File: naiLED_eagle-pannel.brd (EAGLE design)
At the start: 79.5 x 97.8 mm, 378 parts, among them IC1 TCS3414, IC10 TCS3414, IC11 TCS3414, IC12 TCS3414, IC13 TCS3414, IC14 TCS3414, IC15 TCS3414, IC16 TCS3414, IC17 TCS3414, IC18 TCS3414, IC19 TCS3414, IC2 TCS3414, IC20 TCS3414, IC21 TCS3414, IC22 TCS3414, IC23 TCS3414, IC24 TCS3414, IC25 TCS3414, IC26 TCS3414, IC27 TCS3414, IC28 TCS3414, IC29 TCS3414, IC3 TCS3414, IC30 TCS3414, IC31 TCS3414, IC32 TCS3414, IC33 TCS3414, IC34 TCS3414, IC35 TCS3414, IC36 TCS3414, IC37 TCS3414, IC38 TCS3414, IC39 TCS3414, IC4 TCS3414, IC40 TCS3414, IC41 TCS3414, IC42 TCS3414, IC5 TCS3414, IC6 TCS3414, IC7 TCS3414, IC8 TCS3414, IC9 TCS3414, U1 24LC00T-I/OT, U10 ATTINY25-20SSU, U11 24LC00T-I/OT, U12 ATTINY25-20SSU, U13 24LC00T-I/OT, U14 ATTINY25-20SSU, U15 24LC00T-I/OT, U16 ATTINY25-20SSU, U17 24LC00T-I/OT, U18 ATTINY25-20SSU, U19 24LC00T-I/OT, U2 24LC00T-I/OT, U20 ATTINY25-20SSU, U21 24LC00T-I/OT, U22 ATTINY25-20SSU, U23 24LC00T-I/OT, U24 ATTINY25-20SSU, U25 24LC00T-I/OT, U26 ATTINY25-20SSU, U27 24LC00T-I/OT, U28 ATTINY25-20SSU, U29 24LC00T-I/OT, U3 ATTINY25-20SSU, U30 ATTINY25-20SSU, U31 24LC00T-I/OT, U32 ATTINY25-20SSU, U33 24LC00T-I/OT, U34 ATTINY25-20SSU, U35 24LC00T-I/OT, U36 ATTINY25-20SSU, U37 24LC00T-I/OT, U38 ATTINY25-20SSU, U39 24LC00T-I/OT, U4 ATTINY25-20SSU, U40 ATTINY25-20SSU, U41 24LC00T-I/OT, U42 ATTINY25-20SSU, U43 24LC00T-I/OT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

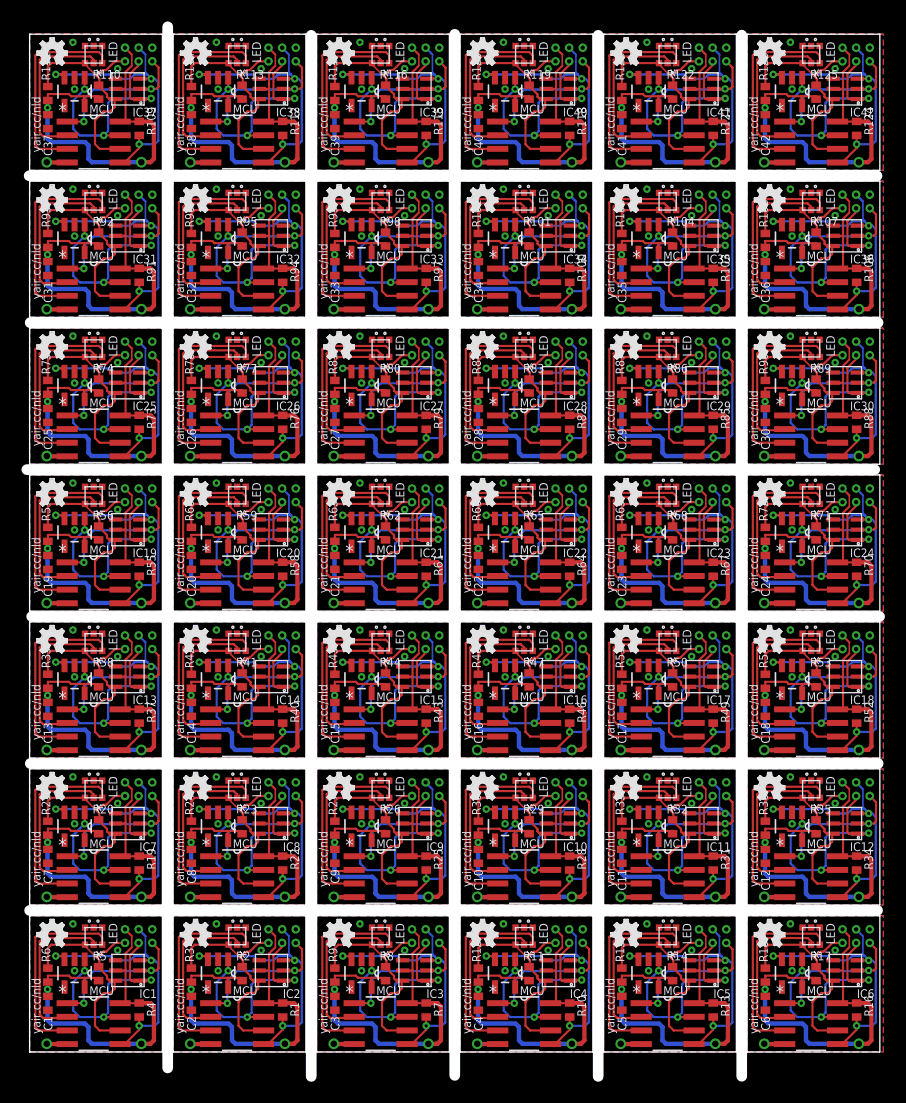
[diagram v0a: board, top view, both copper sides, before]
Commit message: auditing
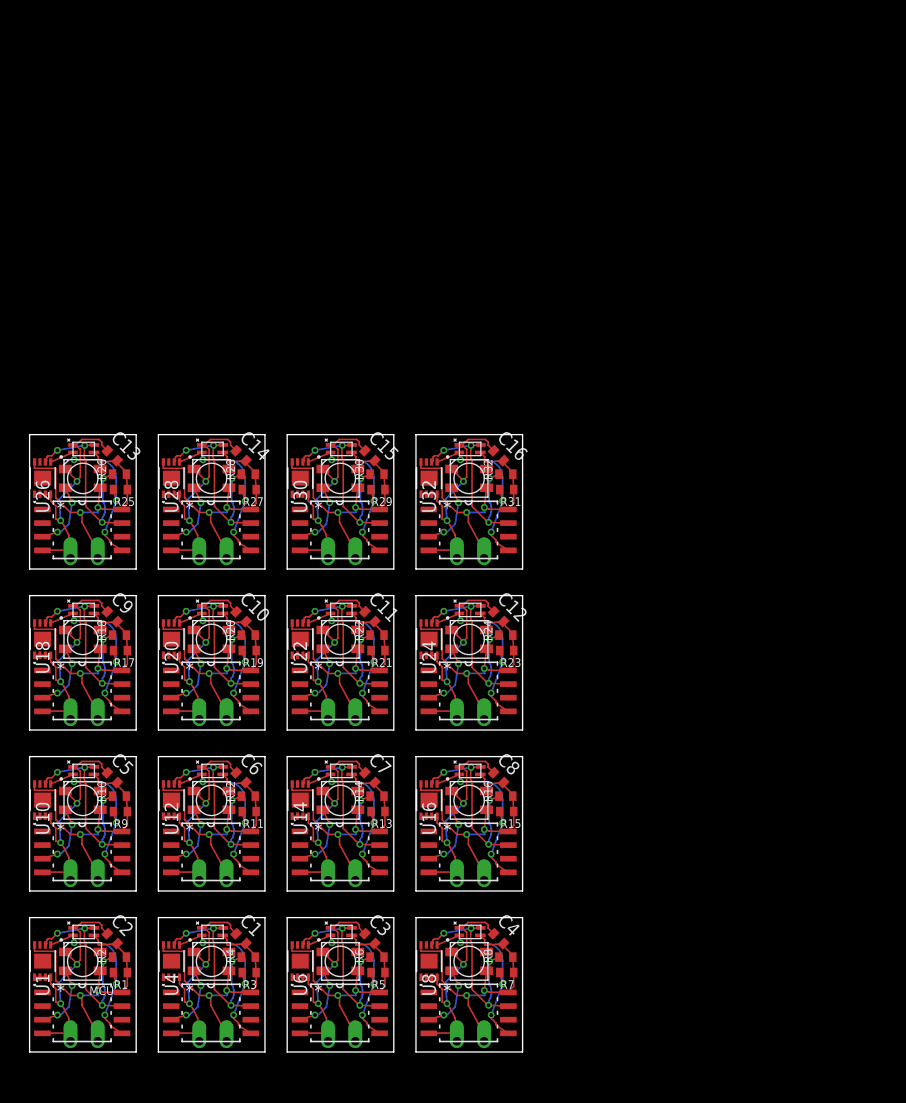
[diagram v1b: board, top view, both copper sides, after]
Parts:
- removed C17, C18, C19, C20, C21, C22, C23, C24, C25, C26, C27, C28, C29, C30, C31, C32, C33, C34, C35, C36, C37, C38, C39, C40, C41, C42: (no value), dp_devices:C402
- removed E$17, E$18, E$19, E$20, E$21, E$22, E$23, E$24, E$25, E$26, E$27, E$28, E$29, E$30, E$31, E$32, E$33, E$34, E$35, E$36, E$37, E$38, E$39, E$40, E$41, E$42: (no value), Logo:OSHW_FILLX100_NOTEXT
- removed IC1, IC10, IC11, IC12, IC13, IC14, IC15, IC16, IC17, IC18, IC19, IC2, IC20, IC21, IC22, IC23, IC24, IC25, IC26, IC27, IC28, IC29, IC3, IC30, IC31, IC32, IC33, IC34, IC35, IC36, IC37, IC38, IC39, IC4, IC40, IC41, IC42, IC5, IC6, IC7, IC8, IC9: TCS3414, yair_r:DFN-6PIN
- removed LED1, LED10, LED11, LED12, LED13, LED14, LED15, LED16, LED17, LED18, LED19, LED2, LED20, LED21, LED22, LED23, LED24, LED25, LED26, LED27, LED28, LED29, LED3, LED30, LED31, LED32, LED33, LED34, LED35, LED36, LED37, LED38, LED39, LED4, LED40, LED41, LED42, LED5, LED6, LED7, LED8, LED9: LED_RGB3, dp_devices:RGBLED
- removed R100, R101, R102, R103, R104, R105, R106, R107, R108, R109, R110, R111, R112, R113, R114, R115, R116, R117, R118, R119, R120, R121, R122, R123, R124, R125, R126, R33, R34, R35, R36, R37, R38, R39, R40, R41, R42, R43, R44, R45, R46, R47, R48, R49, R50, R51, R52, R53, R54, R55, R56, R57, R58, R59, R60, R61, R62, R63, R64, R65, R66, R67, R68, R69, R70, R71, R72, R73, R74, R75, R76, R77, R78, R79, R80, R81, R82, R83, R84, R85, R86, R87, R88, R89, R90, R91, R92, R93, R94, R95, R96, R97, R98, R99: (no value), dp_devices:R402
- removed U33, U35, U37, U39, U41, U43, U45, U47, U49, U51, U53, U55, U57, U59, U61, U63, U65, U67, U69, U71, U73, U75, U77, U79, U81, U83: 24LC00T-I/OT, Microchip-24LCxxx:SOT95P290X145-5N
- removed U34, U36, U38, U40, U42, U44, U46, U48, U50, U52, U54, U56, U58, U60, U62, U64, U66, U68, U70, U72, U74, U76, U78, U80, U82, U84: ATTINY25-20SSU, yair_r:SOIC127P600X175-8N
- added U$1, U$10, U$13, U$16, U$19, U$22, U$25, U$28, U$31, U$34, U$37, U$4, U$40, U$43, U$46, U$7: SK6812MINI, naiLED_eagle:LED-3535
- added U$11, U$14, U$17, U$2, U$20, U$23, U$26, U$29, U$32, U$35, U$38, U$41, U$44, U$47, U$5, U$8: VEML6040, naiLED_eagle:4-TFLGA
- added U$12, U$15, U$18, U$21, U$24, U$27, U$3, U$30, U$33, U$36, U$39, U$42, U$45, U$48, U$6, U$9, VCC, VCC1, VCC10, VCC11, VCC12, VCC13, VCC14, VCC15, VCC2, VCC3, VCC4, VCC5, VCC6, VCC7, VCC8, VCC9: HEADER-1X1, naiLED_eagle:1X1_LONG
- C1, C10, C11, C12, C13, C14, C15, C16, C2, C3, C4, C5, C6, C7, C8, C9: device dp_devices:C402 -> naiLED_eagle:C402
- R1, R10, R11, R12, R13, R14, R15, R16, R17, R18, R19, R2, R20, R21, R22, R23, R24, R25, R26, R27, R28, R29, R3, R30, R31, R32, R4, R5, R6, R7, R8, R9: device dp_devices:R402 -> naiLED_eagle:R402
- U1: value 24LC00T-I/OT -> AT24C256C-MAHL-T; device Microchip-24LCxxx:SOT95P290X145-5N -> naiLED_eagle:8MA2
- U10, U12, U14, U16, U18, U20, U22, U24, U26, U28, U30, U32, U4, U6, U8: value ATTINY25-20SSU -> AT24C256C-MAHL-T; device yair_r:SOIC127P600X175-8N -> naiLED_eagle:8MA2
- U11, U13, U15, U17, U19, U2, U21, U23, U25, U27, U29, U31, U5, U7, U9: value 24LC00T-I/OT -> ATTINY85-20SU; device Microchip-24LCxxx:SOT95P290X145-5N -> naiLED_eagle:SOIC127P798X216-8N
- U3: value ATTINY25-20SSU -> ATTINY85-20SU; device yair_r:SOIC127P600X175-8N -> naiLED_eagle:SOIC127P798X216-8N
- moved R17 71.5 mm to (8.46, 37.4), turned to 0 degrees
- moved R18 68.0 mm to (8.37, 38.8), turned to 0 degrees
- moved U12 63.1 mm to (13.2, 23.5), turned to 90 degrees
- moved U10 61.8 mm to (1.22, 23.5), turned to 90 degrees
- moved U11 55.3 mm to (16.9, 18.6), turned to 0 degrees
- moved U9 54.0 mm to (4.90, 18.6), turned to 0 degrees
- moved C6 53.2 mm to (19.7, 25.6), turned to 315 degrees
- moved C5 51.9 mm to (7.70, 25.6), turned to 315 degrees
- moved E$6 50.8 mm to (18.3, 22.5), flipped to the bottom
- moved E$5 49.5 mm to (6.32, 22.5), flipped to the bottom
- moved R28 47.0 mm to (20.4, 53.8), turned to 0 degrees
- moved R10 46.4 mm to (8.37, 23.8), turned to 0 degrees
- moved R25 45.0 mm to (8.46, 52.4), turned to 0 degrees
- moved U24 41.9 mm to (37.2, 38.5), turned to 90 degrees
- moved R26 41.2 mm to (8.37, 53.8), turned to 0 degrees
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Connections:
- removed net D0/PWM/MOSI/SDA16: IC17.P$3, R49.1, U33.3, U34.5
- removed net D0/PWM/MOSI/SDA17: IC18.P$3, R52.1, U35.3, U36.5
- removed net D0/PWM/MOSI/SDA18: IC19.P$3, R55.1, U37.3, U38.5
- removed net D0/PWM/MOSI/SDA19: IC20.P$3, R58.1, U39.3, U40.5
- removed net D0/PWM/MOSI/SDA20: IC21.P$3, R61.1, U41.3, U42.5
- removed net D0/PWM/MOSI/SDA21: IC22.P$3, R64.1, U43.3, U44.5
- removed net D0/PWM/MOSI/SDA22: IC23.P$3, R67.1, U45.3, U46.5
- removed net D0/PWM/MOSI/SDA23: IC24.P$3, R70.1, U47.3, U48.5
- removed net D0/PWM/MOSI/SDA24: IC25.P$3, R73.1, U49.3, U50.5
- removed net D0/PWM/MOSI/SDA25: IC26.P$3, R76.1, U51.3, U52.5
- removed net D0/PWM/MOSI/SDA26: IC27.P$3, R79.1, U53.3, U54.5
- removed net D0/PWM/MOSI/SDA27: IC28.P$3, R82.1, U55.3, U56.5
- removed net D0/PWM/MOSI/SDA28: IC29.P$3, R85.1, U57.3, U58.5
- removed net D0/PWM/MOSI/SDA29: IC30.P$3, R88.1, U59.3, U60.5
- removed net D0/PWM/MOSI/SDA30: IC31.P$3, R91.1, U61.3, U62.5
- removed net D0/PWM/MOSI/SDA31: IC32.P$3, R94.1, U63.3, U64.5
- removed net D0/PWM/MOSI/SDA32: IC33.P$3, R97.1, U65.3, U66.5
- removed net D0/PWM/MOSI/SDA33: IC34.P$3, R100.1, U67.3, U68.5
- removed net D0/PWM/MOSI/SDA34: IC35.P$3, R103.1, U69.3, U70.5
- removed net D0/PWM/MOSI/SDA35: IC36.P$3, R106.1, U71.3, U72.5
- removed net D0/PWM/MOSI/SDA36: IC37.P$3, R109.1, U73.3, U74.5
- removed net D0/PWM/MOSI/SDA37: IC38.P$3, R112.1, U75.3, U76.5
- removed net D0/PWM/MOSI/SDA38: IC39.P$3, R115.1, U77.3, U78.5
- removed net D0/PWM/MOSI/SDA39: IC40.P$3, R118.1, U79.3, U80.5
- removed net D0/PWM/MOSI/SDA40: IC41.P$3, R121.1, U81.3, U82.5
- removed net D0/PWM/MOSI/SDA41: IC42.P$3, R124.1, U83.3, U84.5
- removed net D1/PWM/MISO16: IC17.P$4, LED17.AG, R50.1, R51.2, U34.6
- removed net D1/PWM/MISO17: IC18.P$4, LED18.AG, R53.1, R54.2, U36.6
- removed net D1/PWM/MISO18: IC19.P$4, LED19.AG, R56.1, R57.2, U38.6
- removed net D1/PWM/MISO19: IC20.P$4, LED20.AG, R59.1, R60.2, U40.6
- removed net D1/PWM/MISO20: IC21.P$4, LED21.AG, R62.1, R63.2, U42.6
- removed net D1/PWM/MISO21: IC22.P$4, LED22.AG, R65.1, R66.2, U44.6
- removed net D1/PWM/MISO22: IC23.P$4, LED23.AG, R68.1, R69.2, U46.6
- removed net D1/PWM/MISO23: IC24.P$4, LED24.AG, R71.1, R72.2, U48.6
- removed net D1/PWM/MISO24: IC25.P$4, LED25.AG, R74.1, R75.2, U50.6
- removed net D1/PWM/MISO25: IC26.P$4, LED26.AG, R77.1, R78.2, U52.6
- removed net D1/PWM/MISO26: IC27.P$4, LED27.AG, R80.1, R81.2, U54.6
- removed net D1/PWM/MISO27: IC28.P$4, LED28.AG, R83.1, R84.2, U56.6
- removed net D1/PWM/MISO28: IC29.P$4, LED29.AG, R86.1, R87.2, U58.6
- removed net D1/PWM/MISO29: IC30.P$4, LED30.AG, R89.1, R90.2, U60.6
- removed net D1/PWM/MISO30: IC31.P$4, LED31.AG, R92.1, R93.2, U62.6
- removed net D1/PWM/MISO31: IC32.P$4, LED32.AG, R95.1, R96.2, U64.6
- removed net D1/PWM/MISO32: IC33.P$4, LED33.AG, R98.1, R99.2, U66.6
- removed net D1/PWM/MISO33: IC34.P$4, LED34.AG, R101.1, R102.2, U68.6
- removed net D1/PWM/MISO34: IC35.P$4, LED35.AG, R104.1, R105.2, U70.6
- removed net D1/PWM/MISO35: IC36.P$4, LED36.AG, R107.1, R108.2, U72.6
- removed net D1/PWM/MISO36: IC37.P$4, LED37.AG, R110.1, R111.2, U74.6
- removed net D1/PWM/MISO37: IC38.P$4, LED38.AG, R113.1, R114.2, U76.6
- removed net D1/PWM/MISO38: IC39.P$4, LED39.AG, R116.1, R117.2, U78.6
- removed net D1/PWM/MISO39: IC40.P$4, LED40.AG, R119.1, R120.2, U80.6
- removed net D1/PWM/MISO40: IC41.P$4, LED41.AG, R122.1, R123.2, U82.6
- removed net D1/PWM/MISO41: IC42.P$4, LED42.AG, R125.1, R126.2, U84.6
- removed net D2/A1/SCK/SCL16: IC17.P$1, U33.1, U34.7
- removed net D2/A1/SCK/SCL17: IC18.P$1, U35.1, U36.7
- removed net D2/A1/SCK/SCL18: IC19.P$1, U37.1, U38.7
- removed net D2/A1/SCK/SCL19: IC20.P$1, U39.1, U40.7
- removed net D2/A1/SCK/SCL20: IC21.P$1, U41.1, U42.7
- removed net D2/A1/SCK/SCL21: IC22.P$1, U43.1, U44.7
- removed net D2/A1/SCK/SCL22: IC23.P$1, U45.1, U46.7
- removed net D2/A1/SCK/SCL23: IC24.P$1, U47.1, U48.7
- removed net D2/A1/SCK/SCL24: IC25.P$1, U49.1, U50.7
- removed net D2/A1/SCK/SCL25: IC26.P$1, U51.1, U52.7
- removed net D2/A1/SCK/SCL26: IC27.P$1, U53.1, U54.7
- removed net D2/A1/SCK/SCL27: IC28.P$1, U55.1, U56.7
- removed net D2/A1/SCK/SCL28: IC29.P$1, U57.1, U58.7
- removed net D2/A1/SCK/SCL29: IC30.P$1, U59.1, U60.7
- removed net D2/A1/SCK/SCL30: IC31.P$1, U61.1, U62.7
- removed net D2/A1/SCK/SCL31: IC32.P$1, U63.1, U64.7
- removed net D2/A1/SCK/SCL32: IC33.P$1, U65.1, U66.7
- removed net D2/A1/SCK/SCL33: IC34.P$1, U67.1, U68.7
- removed net D2/A1/SCK/SCL34: IC35.P$1, U69.1, U70.7
- removed net D2/A1/SCK/SCL35: IC36.P$1, U71.1, U72.7
- removed net D2/A1/SCK/SCL36: IC37.P$1, U73.1, U74.7
- removed net D2/A1/SCK/SCL37: IC38.P$1, U75.1, U76.7
- removed net D2/A1/SCK/SCL38: IC39.P$1, U77.1, U78.7
- removed net D2/A1/SCK/SCL39: IC40.P$1, U79.1, U80.7
- removed net D2/A1/SCK/SCL40: IC41.P$1, U81.1, U82.7
- removed net D2/A1/SCK/SCL41: IC42.P$1, U83.1, U84.7
- removed net D3/A17: LED17.AR, U34.2
- removed net D3/A18: LED18.AR, U36.2
- removed net D3/A19: LED19.AR, U38.2
- removed net D3/A20: LED20.AR, U40.2
- removed net D3/A21: LED21.AR, U42.2
- removed net D3/A22: LED22.AR, U44.2
- removed net D3/A23: LED23.AR, U46.2
- removed net D3/A24: LED24.AR, U48.2
- removed net D3/A25: LED25.AR, U50.2
- removed net D3/A26: LED26.AR, U52.2
- removed net D3/A27: LED27.AR, U54.2
- removed net D3/A28: LED28.AR, U56.2
- removed net D3/A29: LED29.AR, U58.2
- removed net D3/A30: LED30.AR, U60.2
- removed net D3/A31: LED31.AR, U62.2
- removed net D3/A32: LED32.AR, U64.2
- removed net D3/A33: LED33.AR, U66.2
- removed net D3/A34: LED34.AR, U68.2
- removed net D3/A35: LED35.AR, U70.2
- removed net D3/A36: LED36.AR, U72.2
- removed net D3/A37: LED37.AR, U74.2
- removed net D3/A38: LED38.AR, U76.2
- removed net D3/A39: LED39.AR, U78.2
- removed net D3/A40: LED40.AR, U80.2
- removed net D3/A41: LED41.AR, U82.2
- removed net D3/A42: LED42.AR, U84.2
- removed net D4/PWM16: LED17.AB, U34.3
- removed net D4/PWM17: LED18.AB, U36.3
- removed net D4/PWM18: LED19.AB, U38.3
- removed net D4/PWM19: LED20.AB, U40.3
- removed net D4/PWM20: LED21.AB, U42.3
- removed net D4/PWM21: LED22.AB, U44.3
- removed net D4/PWM22: LED23.AB, U46.3
- removed net D4/PWM23: LED24.AB, U48.3
- removed net D4/PWM24: LED25.AB, U50.3
- removed net D4/PWM25: LED26.AB, U52.3
- removed net D4/PWM26: LED27.AB, U54.3
- removed net D4/PWM27: LED28.AB, U56.3
- removed net D4/PWM28: LED29.AB, U58.3
- removed net D4/PWM29: LED30.AB, U60.3
- removed net D4/PWM30: LED31.AB, U62.3
- removed net D4/PWM31: LED32.AB, U64.3
- removed net D4/PWM32: LED33.AB, U66.3
- removed net D4/PWM33: LED34.AB, U68.3
- removed net D4/PWM34: LED35.AB, U70.3
- removed net D4/PWM35: LED36.AB, U72.3
- removed net D4/PWM36: LED37.AB, U74.3
- removed net D4/PWM37: LED38.AB, U76.3
- removed net D4/PWM38: LED39.AB, U78.3
- removed net D4/PWM39: LED40.AB, U80.3
- removed net D4/PWM40: LED41.AB, U82.3
- removed net D4/PWM41: LED42.AB, U84.3
- removed net D5/A0/RESET: IC1.P$2, U3.1
- removed net D5/A0/RESET1: IC2.P$2, U4.1
- removed net D5/A0/RESET10: IC11.P$2, U22.1
- removed net D5/A0/RESET11: IC12.P$2, U24.1
- removed net D5/A0/RESET12: IC13.P$2, U26.1
- removed net D5/A0/RESET13: IC14.P$2, U28.1
- removed net D5/A0/RESET14: IC15.P$2, U30.1
- removed net D5/A0/RESET15: IC16.P$2, U32.1
- removed net D5/A0/RESET16: IC17.P$2, U34.1
- removed net D5/A0/RESET17: IC18.P$2, U36.1
- removed net D5/A0/RESET18: IC19.P$2, U38.1
- removed net D5/A0/RESET19: IC20.P$2, U40.1
- removed net D5/A0/RESET2: IC3.P$2, U6.1
- removed net D5/A0/RESET20: IC21.P$2, U42.1
- removed net D5/A0/RESET21: IC22.P$2, U44.1
- removed net D5/A0/RESET22: IC23.P$2, U46.1
- removed net D5/A0/RESET23: IC24.P$2, U48.1
- removed net D5/A0/RESET24: IC25.P$2, U50.1
- removed net D5/A0/RESET25: IC26.P$2, U52.1
- removed net D5/A0/RESET26: IC27.P$2, U54.1
- removed net D5/A0/RESET27: IC28.P$2, U56.1
- removed net D5/A0/RESET28: IC29.P$2, U58.1
- removed net D5/A0/RESET29: IC30.P$2, U60.1
- removed net D5/A0/RESET3: IC4.P$2, U8.1
- removed net D5/A0/RESET30: IC31.P$2, U62.1
- removed net D5/A0/RESET31: IC32.P$2, U64.1
- removed net D5/A0/RESET32: IC33.P$2, U66.1
- removed net D5/A0/RESET33: IC34.P$2, U68.1
- removed net D5/A0/RESET34: IC35.P$2, U70.1
- removed net D5/A0/RESET35: IC36.P$2, U72.1
- removed net D5/A0/RESET36: IC37.P$2, U74.1
- removed net D5/A0/RESET37: IC38.P$2, U76.1
- removed net D5/A0/RESET38: IC39.P$2, U78.1
- removed net D5/A0/RESET39: IC40.P$2, U80.1
- removed net D5/A0/RESET4: IC5.P$2, U10.1
- removed net D5/A0/RESET40: IC41.P$2, U82.1
- removed net D5/A0/RESET41: IC42.P$2, U84.1
- removed net D5/A0/RESET5: IC6.P$2, U12.1
- removed net D5/A0/RESET6: IC7.P$2, U14.1
- removed net D5/A0/RESET7: IC8.P$2, U16.1
- removed net D5/A0/RESET8: IC9.P$2, U18.1
- removed net D5/A0/RESET9: IC10.P$2, U20.1
- removed net GND16: C17.2, IC17.P$6, LED17.CB, LED17.CG, LED17.CR, U33.2, U34.4
- removed net GND17: C18.2, IC18.P$6, LED18.CB, LED18.CG, LED18.CR, U35.2, U36.4
- removed net GND18: C19.2, IC19.P$6, LED19.CB, LED19.CG, LED19.CR, U37.2, U38.4
- removed net GND19: C20.2, IC20.P$6, LED20.CB, LED20.CG, LED20.CR, U39.2, U40.4
- removed net GND20: C21.2, IC21.P$6, LED21.CB, LED21.CG, LED21.CR, U41.2, U42.4
- removed net GND21: C22.2, IC22.P$6, LED22.CB, LED22.CG, LED22.CR, U43.2, U44.4
- removed net GND22: C23.2, IC23.P$6, LED23.CB, LED23.CG, LED23.CR, U45.2, U46.4
- removed net GND23: C24.2, IC24.P$6, LED24.CB, LED24.CG, LED24.CR, U47.2, U48.4
- removed net GND24: C25.2, IC25.P$6, LED25.CB, LED25.CG, LED25.CR, U49.2, U50.4
- removed net GND25: C26.2, IC26.P$6, LED26.CB, LED26.CG, LED26.CR, U51.2, U52.4
- removed net GND26: C27.2, IC27.P$6, LED27.CB, LED27.CG, LED27.CR, U53.2, U54.4
- removed net GND27: C28.2, IC28.P$6, LED28.CB, LED28.CG, LED28.CR, U55.2, U56.4
- removed net GND28: C29.2, IC29.P$6, LED29.CB, LED29.CG, LED29.CR, U57.2, U58.4
- removed net GND29: C30.2, IC30.P$6, LED30.CB, LED30.CG, LED30.CR, U59.2, U60.4
- removed net GND30: C31.2, IC31.P$6, LED31.CB, LED31.CG, LED31.CR, U61.2, U62.4
- removed net GND31: C32.2, IC32.P$6, LED32.CB, LED32.CG, LED32.CR, U63.2, U64.4
- removed net GND32: C33.2, IC33.P$6, LED33.CB, LED33.CG, LED33.CR, U65.2, U66.4
- removed net GND33: C34.2, IC34.P$6, LED34.CB, LED34.CG, LED34.CR, U67.2, U68.4
- removed net GND34: C35.2, IC35.P$6, LED35.CB, LED35.CG, LED35.CR, U69.2, U70.4
- removed net GND35: C36.2, IC36.P$6, LED36.CB, LED36.CG, LED36.CR, U71.2, U72.4
- removed net GND36: C37.2, IC37.P$6, LED37.CB, LED37.CG, LED37.CR, U73.2, U74.4
- removed net GND37: C38.2, IC38.P$6, LED38.CB, LED38.CG, LED38.CR, U75.2, U76.4
- removed net GND38: C39.2, IC39.P$6, LED39.CB, LED39.CG, LED39.CR, U77.2, U78.4
- removed net GND39: C40.2, IC40.P$6, LED40.CB, LED40.CG, LED40.CR, U79.2, U80.4
- removed net GND40: C41.2, IC41.P$6, LED41.CB, LED41.CG, LED41.CR, U81.2, U82.4
- removed net GND41: C42.2, IC42.P$6, LED42.CB, LED42.CG, LED42.CR, U83.2, U84.4
- removed net VCC16: C17.1, IC17.P$5, R49.2, R50.2, R51.1, U33.5, U34.8
- removed net VCC17: C18.1, IC18.P$5, R52.2, R53.2, R54.1, U35.5, U36.8
- removed net VCC18: C19.1, IC19.P$5, R55.2, R56.2, R57.1, U37.5, U38.8
- removed net VCC19: C20.1, IC20.P$5, R58.2, R59.2, R60.1, U39.5, U40.8
- removed net VCC20: C21.1, IC21.P$5, R61.2, R62.2, R63.1, U41.5, U42.8
- removed net VCC21: C22.1, IC22.P$5, R64.2, R65.2, R66.1, U43.5, U44.8
- removed net VCC22: C23.1, IC23.P$5, R67.2, R68.2, R69.1, U45.5, U46.8
- removed net VCC23: C24.1, IC24.P$5, R70.2, R71.2, R72.1, U47.5, U48.8
- removed net VCC24: C25.1, IC25.P$5, R73.2, R74.2, R75.1, U49.5, U50.8
- removed net VCC25: C26.1, IC26.P$5, R76.2, R77.2, R78.1, U51.5, U52.8
- removed net VCC26: C27.1, IC27.P$5, R79.2, R80.2, R81.1, U53.5, U54.8
- removed net VCC27: C28.1, IC28.P$5, R82.2, R83.2, R84.1, U55.5, U56.8
- removed net VCC28: C29.1, IC29.P$5, R85.2, R86.2, R87.1, U57.5, U58.8
- removed net VCC29: C30.1, IC30.P$5, R88.2, R89.2, R90.1, U59.5, U60.8
- removed net VCC30: C31.1, IC31.P$5, R91.2, R92.2, R93.1, U61.5, U62.8
- removed net VCC31: C32.1, IC32.P$5, R94.2, R95.2, R96.1, U63.5, U64.8
- removed net VCC32: C33.1, IC33.P$5, R97.2, R98.2, R99.1, U65.5, U66.8
- removed net VCC33: C34.1, IC34.P$5, R100.2, R101.2, R102.1, U67.5, U68.8
- removed net VCC34: C35.1, IC35.P$5, R103.2, R104.2, R105.1, U69.5, U70.8
- removed net VCC35: C36.1, IC36.P$5, R106.2, R107.2, R108.1, U71.5, U72.8
- removed net VCC36: C37.1, IC37.P$5, R109.2, R110.2, R111.1, U73.5, U74.8
- removed net VCC37: C38.1, IC38.P$5, R112.2, R113.2, R114.1, U75.5, U76.8
- removed net VCC38: C39.1, IC39.P$5, R115.2, R116.2, R117.1, U77.5, U78.8
- removed net VCC39: C40.1, IC40.P$5, R118.2, R119.2, R120.1, U79.5, U80.8
- removed net VCC40: C41.1, IC41.P$5, R121.2, R122.2, R123.1, U81.5, U82.8
- removed net VCC41: C42.1, IC42.P$5, R124.2, R125.2, R126.1, U83.5, U84.8
- new net NC: U3.1
- new net NC1: U2.1
- new net NC10: U21.1
- new net NC11: U23.1
- new net NC12: U25.1
- new net NC13: U27.1
- new net NC14: U29.1
- new net NC15: U31.1
- new net NC2: U5.1
- new net NC3: U7.1
- new net NC4: U9.1
- new net NC5: U11.1
- new net NC6: U13.1
- new net NC7: U15.1
- new net NC8: U17.1
- new net NC9: U19.1
- net D0/PWM/MOSI/SDA: now also R1.1, U$2.2, U1.5; no longer IC1.P$3, R4.1, U2.3
- net D0/PWM/MOSI/SDA1: now also R3.1, U$5.2, U2.5; no longer IC2.P$3, R1.1, U1.3
- net D0/PWM/MOSI/SDA10: now also R21.1, U$32.2, U21.5; no longer IC11.P$3, R31.1, U21.3
- net D0/PWM/MOSI/SDA11: now also R23.1, U$35.2, U23.5; no longer IC12.P$3, R34.1, U23.3
- net D0/PWM/MOSI/SDA12: now also R25.1, U$38.2, U25.5; no longer IC13.P$3, R37.1, U25.3
- net D0/PWM/MOSI/SDA13: now also R27.1, U$41.2, U27.5; no longer IC14.P$3, R40.1, U27.3
- net D0/PWM/MOSI/SDA14: now also R29.1, U$44.2, U29.5; no longer IC15.P$3, R43.1, U29.3
- net D0/PWM/MOSI/SDA15: now also R31.1, U$47.2, U31.5; no longer IC16.P$3, R46.1, U31.3
- net D0/PWM/MOSI/SDA2: now also R5.1, U$8.2, U5.5; no longer IC3.P$3, R7.1, U5.3
- net D0/PWM/MOSI/SDA3: now also R7.1, U$11.2, U7.5; no longer IC4.P$3, R10.1, U7.3
- net D0/PWM/MOSI/SDA4: now also R9.1, U$14.2, U9.5; no longer IC5.P$3, R13.1, U9.3
- net D0/PWM/MOSI/SDA5: now also R11.1, U$17.2, U11.5; no longer IC6.P$3, R16.1, U11.3
- net D0/PWM/MOSI/SDA6: now also R13.1, U$20.2, U13.5; no longer IC7.P$3, R19.1, U13.3
- net D0/PWM/MOSI/SDA7: now also R15.1, U$23.2, U15.5; no longer IC8.P$3, R22.1, U15.3
- net D0/PWM/MOSI/SDA8: now also R17.1, U$26.2, U17.5; no longer IC9.P$3, R25.1, U17.3
- net D0/PWM/MOSI/SDA9: now also R19.1, U$29.2, U19.5; no longer IC10.P$3, R28.1, U19.3
- net D1/PWM/MISO: no longer IC1.P$4, LED1.AG, R5.1, R6.2
- net D1/PWM/MISO1: now also U2.6; no longer IC2.P$4, LED2.AG, R2.1, R3.2, U4.6
- net D1/PWM/MISO10: now also U21.6; no longer IC11.P$4, LED11.AG, R32.1, R33.2, U22.6
- net D1/PWM/MISO11: now also U23.6; no longer IC12.P$4, LED12.AG, R35.1, R36.2, U24.6
- net D1/PWM/MISO12: now also U25.6; no longer IC13.P$4, LED13.AG, R38.1, R39.2, U26.6
- net D1/PWM/MISO13: now also U27.6; no longer IC14.P$4, LED14.AG, R41.1, R42.2, U28.6
- net D1/PWM/MISO14: now also U29.6; no longer IC15.P$4, LED15.AG, R44.1, R45.2, U30.6
- net D1/PWM/MISO15: now also U31.6; no longer IC16.P$4, LED16.AG, R47.1, R48.2, U32.6
- net D1/PWM/MISO2: now also U5.6; no longer IC3.P$4, LED3.AG, R8.1, R9.2, U6.6
- net D1/PWM/MISO3: now also U7.6; no longer IC4.P$4, LED4.AG, R11.1, R12.2, U8.6
- net D1/PWM/MISO4: now also U9.6; no longer IC5.P$4, LED5.AG, R14.1, R15.2, U10.6
- net D1/PWM/MISO5: now also U11.6; no longer IC6.P$4, LED6.AG, R17.1, R18.2, U12.6
- net D1/PWM/MISO6: now also U13.6; no longer IC7.P$4, LED7.AG, R20.1, R21.2, U14.6
- net D1/PWM/MISO7: now also U15.6; no longer IC8.P$4, LED8.AG, R23.1, R24.2, U16.6
- net D1/PWM/MISO8: now also U17.6; no longer IC9.P$4, LED9.AG, R26.1, R27.2, U18.6
- net D1/PWM/MISO9: now also U19.6; no longer IC10.P$4, LED10.AG, R29.1, R30.2, U20.6
- net D2/A1/SCK/SCL: now also R2.1, U$2.3, U1.6; no longer IC1.P$1, U2.1
- net D2/A1/SCK/SCL1: now also R4.1, U$5.3, U2.7, U4.6; no longer IC2.P$1, U1.1, U4.7
- net D2/A1/SCK/SCL10: now also R22.1, U$32.3, U21.7, U22.6; no longer IC11.P$1, U21.1, U22.7
- net D2/A1/SCK/SCL11: now also R24.1, U$35.3, U23.7, U24.6; no longer IC12.P$1, U23.1, U24.7
- net D2/A1/SCK/SCL12: now also R26.1, U$38.3, U25.7, U26.6; no longer IC13.P$1, U25.1, U26.7
- net D2/A1/SCK/SCL13: now also R28.1, U$41.3, U27.7, U28.6; no longer IC14.P$1, U27.1, U28.7
- net D2/A1/SCK/SCL14: now also R30.1, U$44.3, U29.7, U30.6; no longer IC15.P$1, U29.1, U30.7
- net D2/A1/SCK/SCL15: now also R32.1, U$47.3, U31.7, U32.6; no longer IC16.P$1, U31.1, U32.7
- net D2/A1/SCK/SCL2: now also R6.1, U$8.3, U5.7, U6.6; no longer IC3.P$1, U5.1, U6.7
- net D2/A1/SCK/SCL3: now also R8.1, U$11.3, U7.7, U8.6; no longer IC4.P$1, U7.1, U8.7
- net D2/A1/SCK/SCL4: now also R10.1, U$14.3, U10.6, U9.7; no longer IC5.P$1, U10.7, U9.1
- net D2/A1/SCK/SCL5: now also R12.1, U$17.3, U11.7, U12.6; no longer IC6.P$1, U11.1, U12.7
- net D2/A1/SCK/SCL6: now also R14.1, U$20.3, U13.7, U14.6; no longer IC7.P$1, U13.1, U14.7
- net D2/A1/SCK/SCL7: now also R16.1, U$23.3, U15.7, U16.6; no longer IC8.P$1, U15.1, U16.7
- net D2/A1/SCK/SCL8: now also R18.1, U$26.3, U17.7, U18.6; no longer IC9.P$1, U17.1, U18.7
- net D2/A1/SCK/SCL9: now also R20.1, U$29.3, U19.7, U20.6; no longer IC10.P$1, U19.1, U20.7
- net D3/A1: now also U2.2; no longer LED2.AR, U4.2
- net D3/A10: now also U19.2; no longer LED10.AR, U20.2
- net D3/A11: now also U21.2; no longer LED11.AR, U22.2
- net D3/A12: now also U23.2; no longer LED12.AR, U24.2
- net D3/A13: now also U25.2; no longer LED13.AR, U26.2
- net D3/A14: now also U27.2; no longer LED14.AR, U28.2
- net D3/A15: now also U29.2; no longer LED15.AR, U30.2
- net D3/A16: now also U31.2; no longer LED16.AR, U32.2
- net D3/A2: now also U5.2; no longer LED3.AR, U6.2
- net D3/A3: no longer LED1.AR
- net D3/A4: now also U7.2; no longer LED4.AR, U8.2
- net D3/A5: now also U9.2; no longer LED5.AR, U10.2
- net D3/A6: now also U11.2; no longer LED6.AR, U12.2
- net D3/A7: now also U13.2; no longer LED7.AR, U14.2
- net D3/A8: now also U15.2; no longer LED8.AR, U16.2
- net D3/A9: now also U17.2; no longer LED9.AR, U18.2
- net D4/PWM: now also U$1.2; no longer LED1.AB
- net D4/PWM1: now also U$4.2, U2.3; no longer LED2.AB, U4.3
- net D4/PWM10: now also U$31.2, U21.3; no longer LED11.AB, U22.3
- net D4/PWM11: now also U$34.2, U23.3; no longer LED12.AB, U24.3
- net D4/PWM12: now also U$37.2, U25.3; no longer LED13.AB, U26.3
- net D4/PWM13: now also U$40.2, U27.3; no longer LED14.AB, U28.3
- net D4/PWM14: now also U$43.2, U29.3; no longer LED15.AB, U30.3
- net D4/PWM15: now also U$46.2, U31.3; no longer LED16.AB, U32.3
- net D4/PWM2: now also U$7.2, U5.3; no longer LED3.AB, U6.3
- net D4/PWM3: now also U$10.2, U7.3; no longer LED4.AB, U8.3
- net D4/PWM4: now also U$13.2, U9.3; no longer LED5.AB, U10.3
- net D4/PWM5: now also U$16.2, U11.3; no longer LED6.AB, U12.3
- net D4/PWM6: now also U$19.2, U13.3; no longer LED7.AB, U14.3
- net D4/PWM7: now also U$22.2, U15.3; no longer LED8.AB, U16.3
- net D4/PWM8: now also U$25.2, U17.3; no longer LED9.AB, U18.3
- net D4/PWM9: now also U$28.2, U19.3; no longer LED10.AB, U20.3
- net GND: now also C2.1, U$1.1, U$2.1, U$3.P$1, U1.1, U1.2, U1.3, U1.4; no longer C1.2, IC1.P$6, LED1.CB, LED1.CG, LED1.CR, U2.2
- net GND1: now also C1.1, U$4.1, U$5.1, U$6.P$1, U2.4, U4.1, U4.2, U4.3; no longer C2.2, IC2.P$6, LED2.CB, LED2.CG, LED2.CR, U1.2
- net GND10: now also C11.1, U$31.1, U$32.1, U$33.P$1, U21.4, U22.1, U22.2, U22.3; no longer C11.2, IC11.P$6, LED11.CB, LED11.CG, LED11.CR, U21.2
- net GND11: now also C12.1, U$34.1, U$35.1, U$36.P$1, U23.4, U24.1, U24.2, U24.3; no longer C12.2, IC12.P$6, LED12.CB, LED12.CG, LED12.CR, U23.2
- net GND12: now also C13.1, U$37.1, U$38.1, U$39.P$1, U25.4, U26.1, U26.2, U26.3; no longer C13.2, IC13.P$6, LED13.CB, LED13.CG, LED13.CR, U25.2
- net GND13: now also C14.1, U$40.1, U$41.1, U$42.P$1, U27.4, U28.1, U28.2, U28.3; no longer C14.2, IC14.P$6, LED14.CB, LED14.CG, LED14.CR, U27.2
- net GND14: now also C15.1, U$43.1, U$44.1, U$45.P$1, U29.4, U30.1, U30.2, U30.3; no longer C15.2, IC15.P$6, LED15.CB, LED15.CG, LED15.CR, U29.2
- net GND15: now also C16.1, U$46.1, U$47.1, U$48.P$1, U31.4, U32.1, U32.2, U32.3; no longer C16.2, IC16.P$6, LED16.CB, LED16.CG, LED16.CR, U31.2
- net GND2: now also C3.1, U$7.1, U$8.1, U$9.P$1, U5.4, U6.1, U6.2, U6.3; no longer C3.2, IC3.P$6, LED3.CB, LED3.CG, LED3.CR, U5.2
- net GND3: now also C4.1, U$10.1, U$11.1, U$12.P$1, U7.4, U8.1, U8.2, U8.3; no longer C4.2, IC4.P$6, LED4.CB, LED4.CG, LED4.CR, U7.2
- net GND4: now also C5.1, U$13.1, U$14.1, U$15.P$1, U10.1, U10.2, U10.3, U9.4; no longer C5.2, IC5.P$6, LED5.CB, LED5.CG, LED5.CR, U9.2
- net GND5: now also C6.1, U$16.1, U$17.1, U$18.P$1, U11.4, U12.1, U12.2, U12.3; no longer C6.2, IC6.P$6, LED6.CB, LED6.CG, LED6.CR, U11.2
- net GND6: now also C7.1, U$19.1, U$20.1, U$21.P$1, U13.4, U14.1, U14.2, U14.3; no longer C7.2, IC7.P$6, LED7.CB, LED7.CG, LED7.CR, U13.2
- net GND7: now also C8.1, U$22.1, U$23.1, U$24.P$1, U15.4, U16.1, U16.2, U16.3; no longer C8.2, IC8.P$6, LED8.CB, LED8.CG, LED8.CR, U15.2
- net GND8: now also C9.1, U$25.1, U$26.1, U$27.P$1, U17.4, U18.1, U18.2, U18.3; no longer C9.2, IC9.P$6, LED9.CB, LED9.CG, LED9.CR, U17.2
- net GND9: now also C10.1, U$28.1, U$29.1, U$30.P$1, U19.4, U20.1, U20.2, U20.3; no longer C10.2, IC10.P$6, LED10.CB, LED10.CG, LED10.CR, U19.2
- net VCC: now also C2.2, R1.2, R2.2, U$1.3, U$2.4, U1.8, VCC.P$1; no longer C1.1, IC1.P$5, R4.2, R5.2, R6.1, U2.5
- net VCC1: now also C1.2, R3.2, R4.2, U$4.3, U$5.4, U2.8, VCC1.P$1; no longer C2.1, IC2.P$5, R1.2, R2.2, R3.1, U1.5
- net VCC10: now also C11.2, R21.2, R22.2, U$31.3, U$32.4, U21.8, VCC10.P$1; no longer C11.1, IC11.P$5, R31.2, R32.2, R33.1, U21.5
- net VCC11: now also C12.2, R23.2, R24.2, U$34.3, U$35.4, U23.8, VCC11.P$1; no longer C12.1, IC12.P$5, R34.2, R35.2, R36.1, U23.5
- net VCC12: now also C13.2, R25.2, R26.2, U$37.3, U$38.4, U25.8, VCC12.P$1; no longer C13.1, IC13.P$5, R37.2, R38.2, R39.1, U25.5
- net VCC13: now also C14.2, R27.2, R28.2, U$40.3, U$41.4, U27.8, VCC13.P$1; no longer C14.1, IC14.P$5, R40.2, R41.2, R42.1, U27.5
- net VCC14: now also C15.2, R29.2, R30.2, U$43.3, U$44.4, U29.8, VCC14.P$1; no longer C15.1, IC15.P$5, R43.2, R44.2, R45.1, U29.5
- net VCC15: now also C16.2, R31.2, R32.2, U$46.3, U$47.4, U31.8, VCC15.P$1; no longer C16.1, IC16.P$5, R46.2, R47.2, R48.1, U31.5
- net VCC2: now also C3.2, R5.2, R6.2, U$7.3, U$8.4, U5.8, VCC2.P$1; no longer C3.1, IC3.P$5, R7.2, R8.2, R9.1, U5.5
- net VCC3: now also C4.2, R7.2, R8.2, U$10.3, U$11.4, U7.8, VCC3.P$1; no longer C4.1, IC4.P$5, R10.2, R11.2, R12.1, U7.5
- net VCC4: now also C5.2, R10.2, R9.2, U$13.3, U$14.4, U9.8, VCC4.P$1; no longer C5.1, IC5.P$5, R13.2, R14.2, R15.1, U9.5
- net VCC5: now also C6.2, R11.2, R12.2, U$16.3, U$17.4, U11.8, VCC5.P$1; no longer C6.1, IC6.P$5, R16.2, R17.2, R18.1, U11.5
- net VCC6: now also C7.2, R13.2, R14.2, U$19.3, U$20.4, U13.8, VCC6.P$1; no longer C7.1, IC7.P$5, R19.2, R20.2, R21.1, U13.5
- net VCC7: now also C8.2, R15.2, R16.2, U$22.3, U$23.4, U15.8, VCC7.P$1; no longer C8.1, IC8.P$5, R22.2, R23.2, R24.1, U15.5
- net VCC8: now also C9.2, R17.2, R18.2, U$25.3, U$26.4, U17.8, VCC8.P$1; no longer C9.1, IC9.P$5, R25.2, R26.2, R27.1, U17.5
- net VCC9: now also C10.2, R19.2, R20.2, U$28.3, U$29.4, U19.8, VCC9.P$1; no longer C10.1, IC10.P$5, R28.2, R29.2, R30.1, U19.5
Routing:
- net VCC23: track 37.9 -> 0.00 mm, vias 3 -> 0
- net VCC35: track 37.9 -> 0.00 mm, vias 3 -> 0
- net VCC17: track 37.9 -> 0.00 mm, vias 3 -> 0
- net VCC41: track 37.9 -> 0.00 mm, vias 3 -> 0
- net VCC29: track 37.9 -> 0.00 mm, vias 3 -> 0
- net VCC21: track 37.9 -> 0.00 mm, vias 3 -> 0
- net VCC16: track 37.9 -> 0.00 mm, vias 3 -> 0
- net VCC22: track 37.9 -> 0.00 mm, vias 3 -> 0
- net VCC20: track 37.9 -> 0.00 mm, vias 3 -> 0
- net VCC19: track 37.9 -> 0.00 mm, vias 3 -> 0
- net VCC18: track 37.9 -> 0.00 mm, vias 3 -> 0
- net VCC37: track 37.9 -> 0.00 mm, vias 3 -> 0
- net VCC33: track 37.9 -> 0.00 mm, vias 3 -> 0
- net VCC31: track 37.9 -> 0.00 mm, vias 3 -> 0
- net VCC40: track 37.9 -> 0.00 mm, vias 3 -> 0
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- removed copper zone on layer 1, net GND
- removed copper zone on layer 16, net GND
- removed copper zone on layer 1, net GND1
- removed copper zone on layer 16, net GND1
- removed copper zone on layer 1, net GND10
- removed copper zone on layer 16, net GND10
- removed copper zone on layer 1, net GND11
- removed copper zone on layer 16, net GND11
- removed copper zone on layer 1, net GND12
- removed copper zone on layer 16, net GND12
- removed copper zone on layer 1, net GND13
- removed copper zone on layer 16, net GND13
- removed copper zone on layer 1, net GND14
- removed copper zone on layer 16, net GND14
- removed copper zone on layer 1, net GND15
- removed copper zone on layer 16, net GND15
- removed copper zone on layer 1, net GND16
- removed copper zone on layer 16, net GND16
- removed copper zone on layer 1, net GND17
- removed copper zone on layer 16, net GND17
- removed copper zone on layer 1, net GND18
- removed copper zone on layer 16, net GND18
- removed copper zone on layer 1, net GND19
- removed copper zone on layer 16, net GND19
- removed copper zone on layer 1, net GND2
- removed copper zone on layer 16, net GND2
- removed copper zone on layer 1, net GND20
- removed copper zone on layer 16, net GND20
- removed copper zone on layer 1, net GND21
- removed copper zone on layer 16, net GND21
- removed copper zone on layer 1, net GND22
- removed copper zone on layer 16, net GND22
- removed copper zone on layer 1, net GND23
- removed copper zone on layer 16, net GND23
- removed copper zone on layer 1, net GND24
- removed copper zone on layer 16, net GND24
- removed copper zone on layer 1, net GND25
- removed copper zone on layer 16, net GND25
- removed copper zone on layer 1, net GND26
- removed copper zone on layer 16, net GND26
- removed copper zone on layer 1, net GND27
- removed copper zone on layer 16, net GND27
- removed copper zone on layer 1, net GND28
- removed copper zone on layer 16, net GND28
- removed copper zone on layer 1, net GND29
- removed copper zone on layer 16, net GND29
- removed copper zone on layer 1, net GND3
- removed copper zone on layer 16, net GND3
- removed copper zone on layer 1, net GND30
- removed copper zone on layer 16, net GND30
- removed copper zone on layer 1, net GND31
- removed copper zone on layer 16, net GND31
- removed copper zone on layer 1, net GND32
- removed copper zone on layer 16, net GND32
- removed copper zone on layer 1, net GND33
- removed copper zone on layer 16, net GND33
- removed copper zone on layer 1, net GND34
- removed copper zone on layer 16, net GND34
- removed copper zone on layer 1, net GND35
- removed copper zone on layer 16, net GND35
- removed copper zone on layer 1, net GND36
- removed copper zone on layer 16, net GND36
- removed copper zone on layer 1, net GND37
- removed copper zone on layer 16, net GND37
- removed copper zone on layer 1, net GND38
- removed copper zone on layer 16, net GND38
- removed copper zone on layer 1, net GND39
- removed copper zone on layer 16, net GND39
- removed copper zone on layer 1, net GND4
- removed copper zone on layer 16, net GND4
- removed copper zone on layer 1, net GND40
- removed copper zone on layer 16, net GND40
- removed copper zone on layer 1, net GND41
- removed copper zone on layer 16, net GND41
- removed copper zone on layer 1, net GND5
- removed copper zone on layer 16, net GND5
- removed copper zone on layer 1, net GND6
- removed copper zone on layer 16, net GND6
- removed copper zone on layer 1, net GND7
- removed copper zone on layer 16, net GND7
- removed copper zone on layer 1, net GND8
- removed copper zone on layer 16, net GND8
- removed copper zone on layer 1, net GND9
- removed copper zone on layer 16, net GND9
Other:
- board size 79.5 x 97.8 mm -> 45.9 x 57.5 mm
- board text removed: "LED"
